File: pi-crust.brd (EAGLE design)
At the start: 43.7 x 40.4 mm, 19 parts

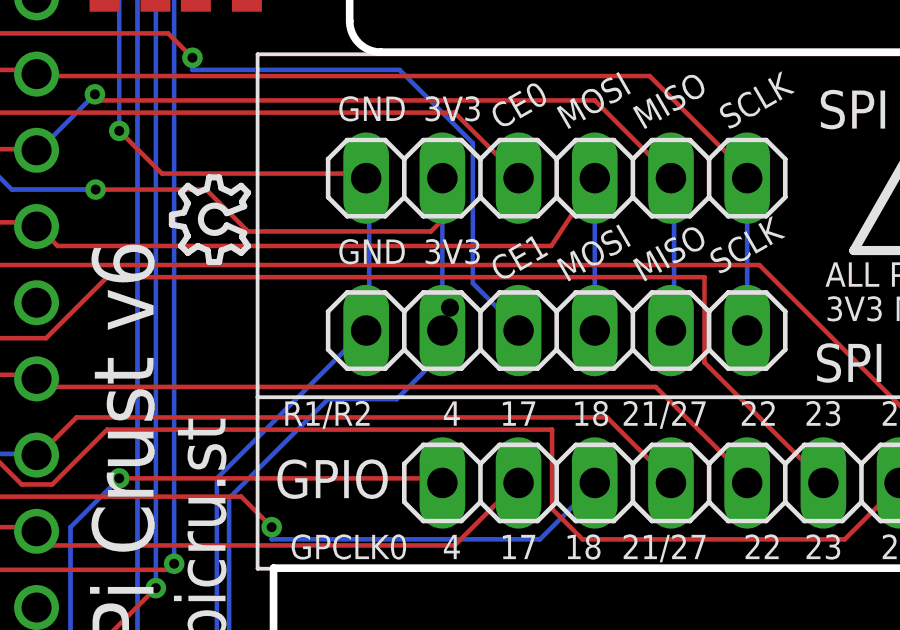
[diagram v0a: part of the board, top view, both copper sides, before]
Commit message: Minor changes..
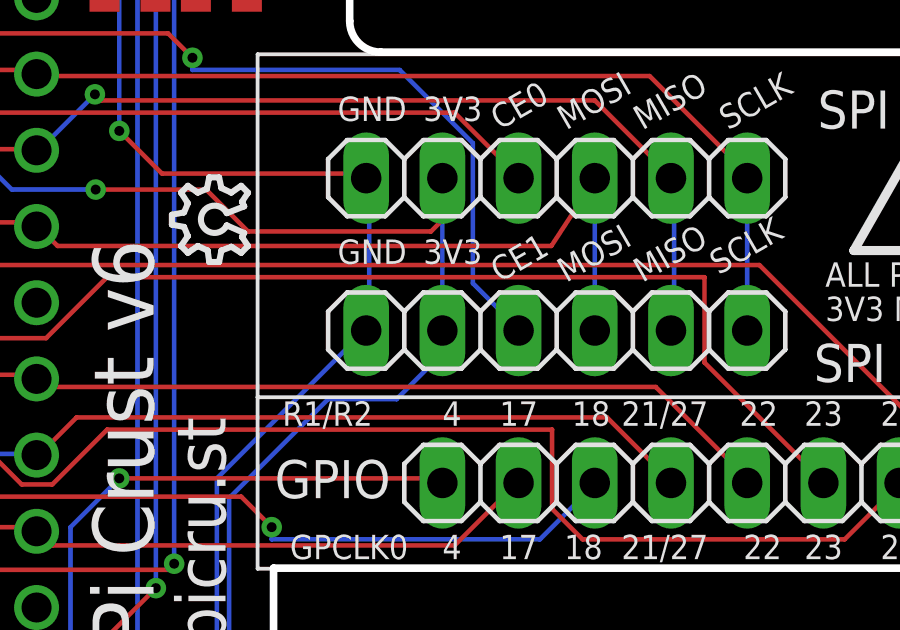
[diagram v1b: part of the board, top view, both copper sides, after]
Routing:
- net 3V3: track 81.0 -> 80.7 mm, vias 3 -> 2
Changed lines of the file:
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@@
 <wire x1="8.343" y1="38.1" x2="8.382" y2="38.735" width="0.1524" layer="1"/>
 <wire x1="25.4" y1="21.59" x2="25.654" y2="21.59" width="0.1524" layer="1"/>
-<wire x1="25.654" y1="21.59" x2="25.654" y2="22.352" width="0.1524" layer="1"/>
-<via x="25.654" y="22.352" extent="1-16" drill="0.6"/>
-<wire x1="25.654" y1="22.352" x2="25.4" y2="22.352" width="0.1524" layer="16"/>
 <wire x1="25.4" y1="22.352" x2="25.4" y2="26.67" width="0.1524" layer="16"/>
 <wire x1="20.32" y1="2.54" x2="20.32" y2="1.016" width="0.1524" layer="16"/>
@@
 <wire x1="25.019" y1="24.892" x2="25.4" y2="25.273" width="0.1524" layer="1"/>
 <wire x1="25.4" y1="25.273" x2="25.4" y2="26.67" width="0.1524" layer="1"/>
+<wire x1="25.4" y1="22.352" x2="25.4" y2="21.59" width="0.4064" layer="16"/>
 <wire x1="6.604" y1="36.8046" x2="6.858" y2="36.8554" width="0" layer="19" extent="1-16"/>
 </signal>
